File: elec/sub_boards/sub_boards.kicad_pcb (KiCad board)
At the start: 2 copper layers, 65.3 x 47.4 mm, 16 parts, among them J1 Conn_01x10, J5 PSR-41253-06O, J6 PSR-41253-06O, J8 Conn_01x07_Pin, SW1 TVBP06-B043CB-B, SW2 TVBP06-B043CB-B, U10 AS5047D, U9 AS5047D

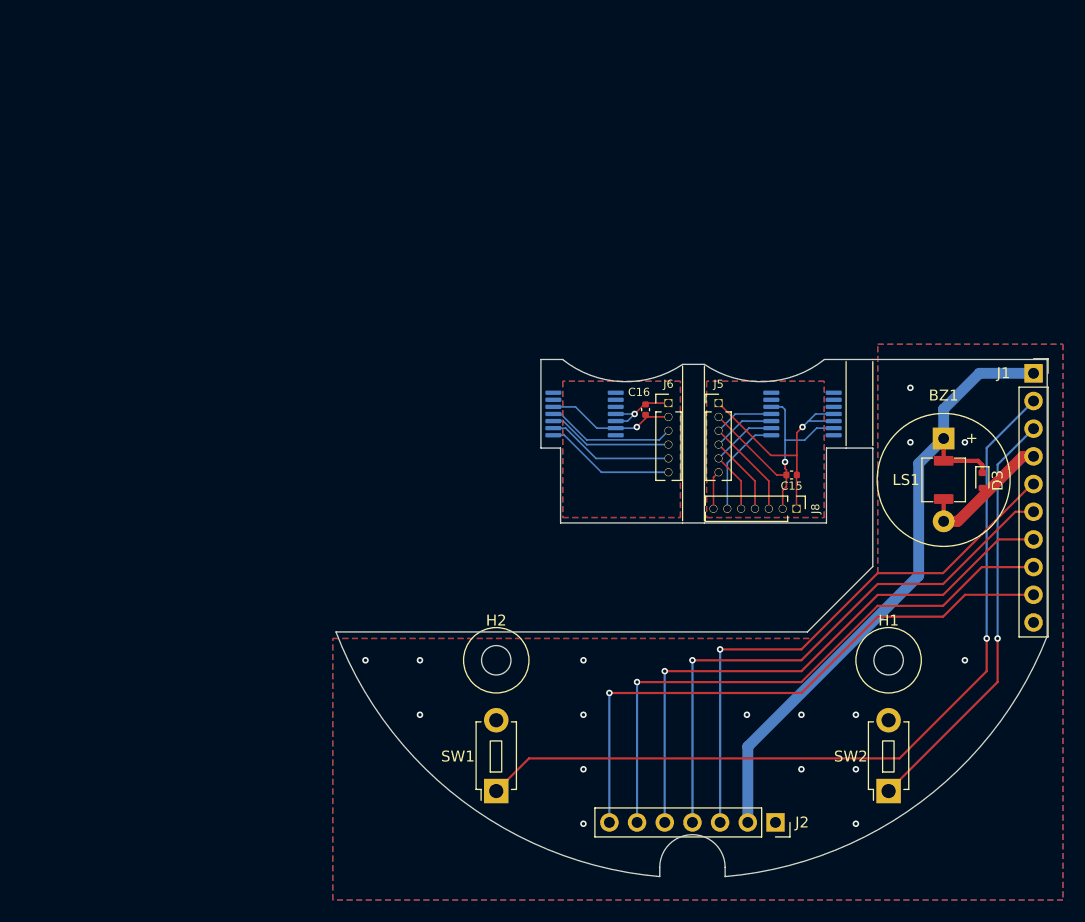
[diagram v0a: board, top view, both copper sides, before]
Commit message: 新エンコーダ基板のアートワーク作業中
Signed-off-by: Kazuki Iida <elkel53930@gmail.com>
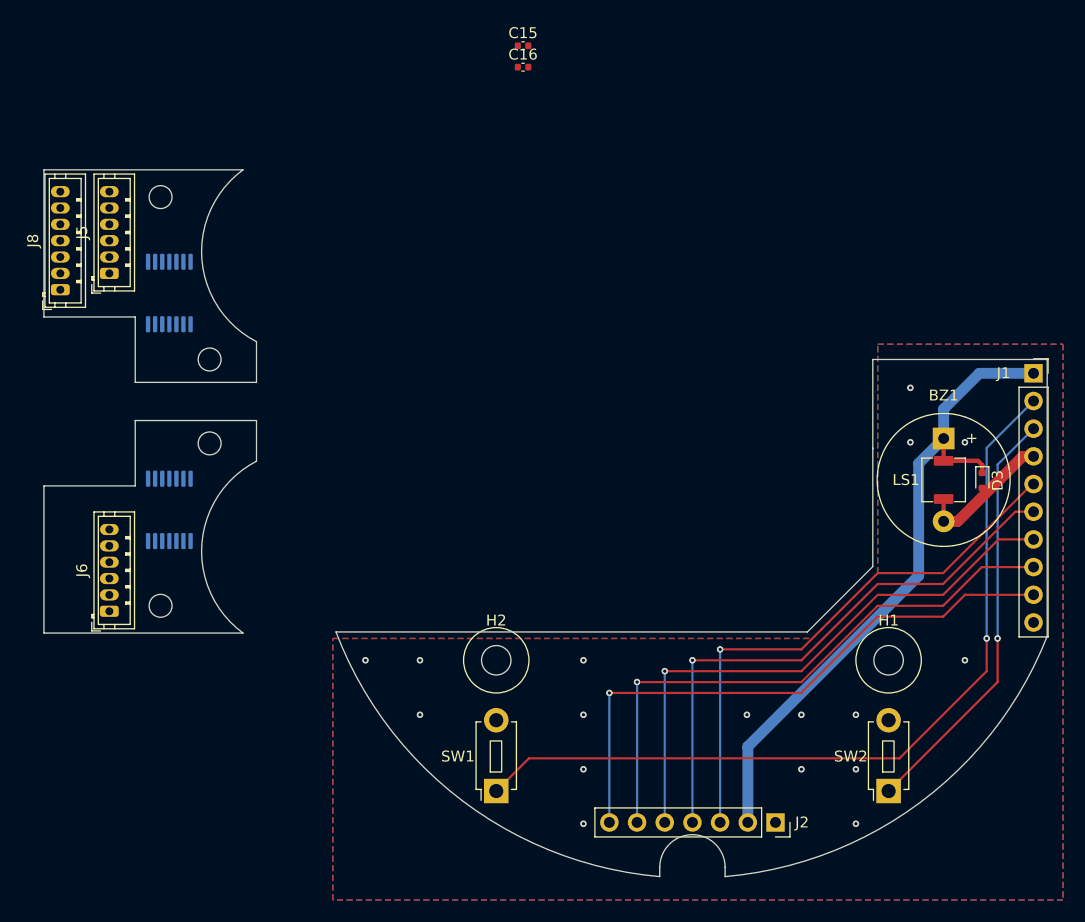
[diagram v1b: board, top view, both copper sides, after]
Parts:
- added H3: M2, MountingHole:MountingHole_2.1mm, F.Cu at (101.2, 72.5)
- added H4: M2, MountingHole:MountingHole_2.1mm, F.Cu at (105.7, 87.4)
- added H5: M2, MountingHole:MountingHole_2.1mm, F.Cu at (105.7, 95.1)
- added H6: M2, MountingHole:MountingHole_2.1mm, F.Cu at (101.2, 110.0)
- J5, J6: footprint Connector_PinHeader_1.27mm:PinHeader_1x06_P1.27mm_Vertical -> Connector_JST:JST_ZH_B6B-ZR_1x06_P1.50mm_Vertical
- J8: footprint Connector_PinHeader_1.27mm:PinHeader_1x07_P1.27mm_Vertical -> Connector_JST:JST_ZH_B7B-ZR_1x07_P1.50mm_Vertical
- moved J8 70.5 mm to (92.0, 81.0), turned to 90 degrees
- moved U9 59.2 mm to (102.0, 81.3), turned to 90 degrees
- moved J5 57.2 mm to (96.5, 79.5), turned to 90 degrees
- moved J6 54.7 mm to (96.5, 110.5), turned to 90 degrees
- moved C15 46.5 mm to (134.5, 58.6)
- moved U10 39.1 mm to (102.0, 101.2), turned to 90 degrees
- moved C16 33.4 mm to (134.5, 60.6), turned to 0 degrees
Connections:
- J6 pad 1: /ENCR__3V3 -> /ENCR_CS_R
- J6 pad 2: /ENCR_GND -> unconnected-(J6-Pin_2-Pad2)
- J6 pad 3: /ENCR_MOSI -> /ENCR_MISO
- J6 pad 4: /ENCR_MISO -> /ENCR_MOSI
- J6 pad 5: /ENCR_SCK -> /ENCR_GND
- J6 pad 6: /ENCR_CS_R -> /ENCR__3V3
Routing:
- net /ENCL_GND: track 24.0 -> 0.00 mm, vias 1 -> 0
- net /ENCL__3V3: track 22.6 -> 0.00 mm, vias 1 -> 0
- net /ENCL_MOSI: track 14.5 -> 0.00 mm
- net /ENCL_MISO: track 13.0 -> 0.00 mm
- net /ENCR_GND: track 12.1 -> 0.00 mm, vias 1 -> 0
- net /ENCR_CS_R: track 12.0 -> 0.00 mm
- net /ENCR_MOSI: track 11.9 -> 0.00 mm
- net /ENCR_SCK: track 11.7 -> 0.00 mm
- net /ENCL_SCK: track 11.5 -> 0.00 mm
- net /ENCR_MISO: track 11.5 -> 0.00 mm
- net /ENCL_CS_L: track 9.29 -> 0.00 mm
- net /ENCR__3V3: track 7.26 -> 0.00 mm, vias 1 -> 0
- net /ENCL_CS_R: track 3.54 -> 0.00 mm
- removed copper zone on B.Cu, net /ENCL_GND
- removed copper zone on F.Cu, net /ENCL_GND
- removed copper zone on B.Cu, net /ENCR_GND
- removed copper zone on F.Cu, net /ENCR_GND
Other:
- board size 65.3 x 47.4 mm -> 92 x 64.8 mm
